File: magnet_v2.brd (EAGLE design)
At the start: 45.7 x 45.7 mm, 30 parts, among them U1 IN100, U2 SGP40-D-R4, U3 BME280, U4 BME280, U5 SGP40-D-R4, Y1 CX3225SB26000D0FLJCC, Y2 ECS-.327-12.5-16-TR

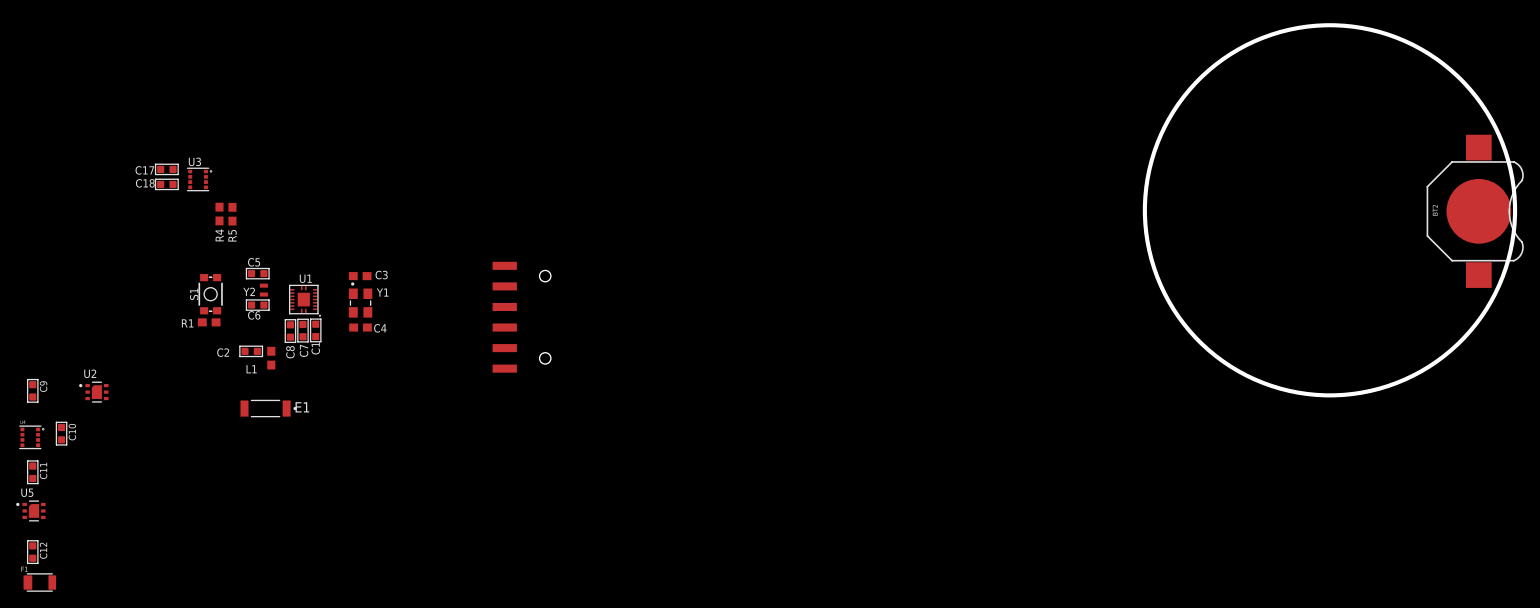
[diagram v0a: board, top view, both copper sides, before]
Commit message: Update magnet_v2.brd
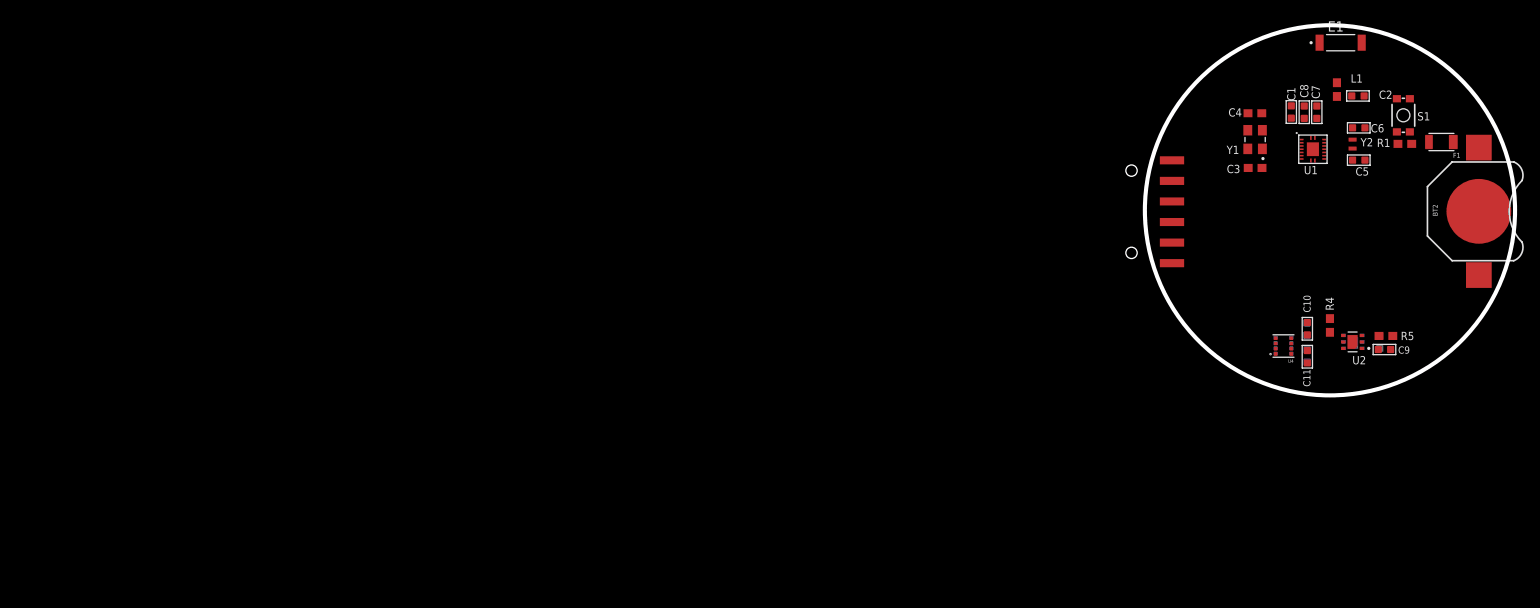
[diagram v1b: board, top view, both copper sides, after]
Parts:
- moved F1 181.5 mm to (36.6, 31.3), turned to 180 degrees
- moved C12 168.4 mm to (29.0, 6.55), flipped to the bottom, turned to 180 degrees
- moved C9 167.0 mm to (29.6, 5.66), turned to 270 degrees
- moved U5 164.2 mm to (25.7, 6.60), flipped to the bottom
- moved C11 158.1 mm to (20.1, 4.78), turned to 180 degrees
- moved U2 155.2 mm to (25.7, 6.60), turned to 180 degrees
- moved U4 155.2 mm to (17.1, 6.10), turned to 180 degrees
- moved C10 154.4 mm to (20.1, 8.23)
- moved R1 149.3 mm to (32.1, 31.1), turned to 0 degrees
- moved S1 149.0 mm to (31.9, 34.6), turned to 270 degrees
- moved R5 143.3 mm to (29.8, 7.34), turned to 0 degrees
- moved C17 142.7 mm to (20.0, 4.88), flipped to the bottom, turned to 180 degrees
- moved C18 141.9 mm to (20.0, 8.18), flipped to the bottom, turned to 0 degrees
- moved C2 140.3 mm to (26.3, 37.0), turned to 90 degrees
- moved E1 140.3 mm to (24.2, 43.6), turned to 0 degrees
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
